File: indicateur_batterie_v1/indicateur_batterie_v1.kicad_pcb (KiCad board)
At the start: 2 copper layers, 28.5 x 16.5 mm, 13 parts, among them J1 Conn_01x02_Pin, Q1 Q_PMOS_GSD, U1 ATtiny412-SS, U3 MCP1802x-xx02xOT

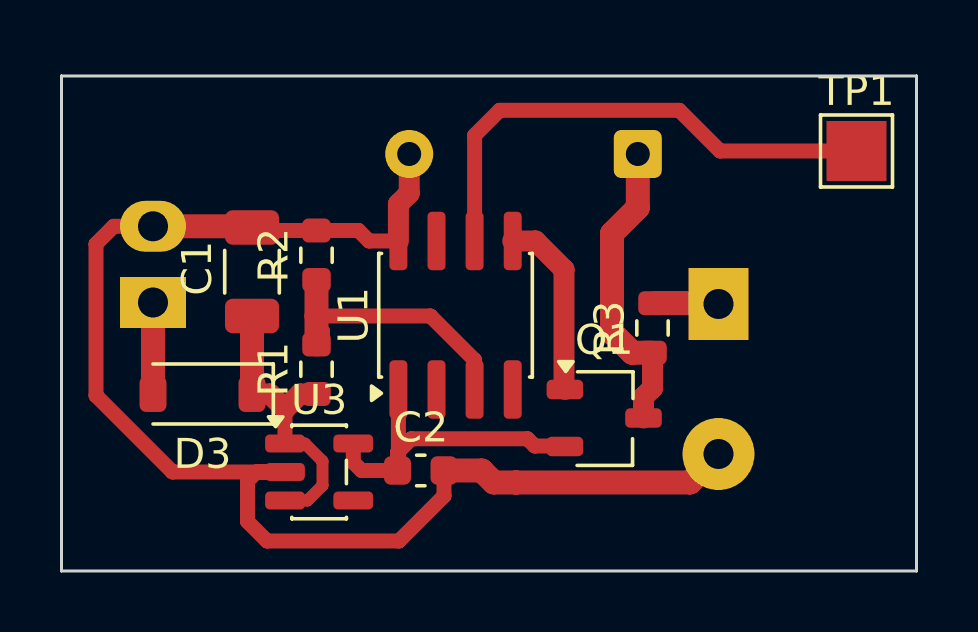
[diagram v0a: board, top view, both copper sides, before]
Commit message: changement déclanchement télécomande
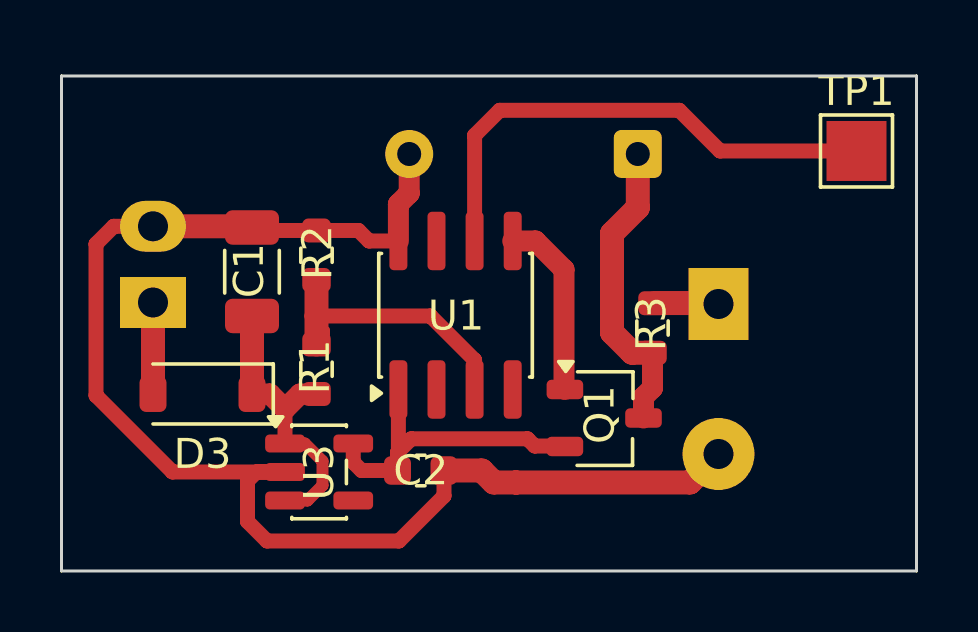
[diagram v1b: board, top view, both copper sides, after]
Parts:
- D3: value D_Schottky -> BAT54W D_Schottky
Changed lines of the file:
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@@
 		(tenting front back)
 		(pcbplotparams
-			(layerselection 0x00000000_00000000_55555555_55555551)
-			(plot_on_all_layers_selection 0x00000000_00000000_00000000_02000000)
+			(layerselection 0x00000000_00000000_55555555_57555550)
+			(plot_on_all_layers_selection 0x00000000_00000000_00000008_00000202)
 			(disableapertmacros no)
 			(usegerberextensions no)
@@
 			(subtractmaskfromsilk no)
 			(outputformat 4)
-			(mirror yes)
+			(mirror no)
 			(drillshape 1)
 			(scaleselection 1)
@@
 			)
 		)
-		(property "Value" "D_Schottky"
-			(at 0 2.1 0)
+		(property "Value" "BAT54W D_Schottky"
+			(at 9.2 0.1 0)
 			(layer "F.Fab")
 			(effects
@@
 		(tags "SOIC SO")
 		(property "Reference" "U1"
-			(at 0 -3.4 90)
+			(at -0.015 0.015 180)
 			(layer "F.SilkS")
 			(effects
@@
 		)
 		(property "Value" "ATtiny412-SS"
-			(at 0 3.4 90)
+			(at -9.265 1.705 90)
 			(layer "F.Fab")
 			(effects
@@
 		(tags "resistor")
 		(property "Reference" "R3"
-			(at 0 -1.43 90)
+			(at 0.14 -0.04 90)
 			(layer "F.SilkS")
 			(effects
@@
 		)
 		(property "Value" "0"
-			(at 0 1.43 90)
+			(at 2.13 0.04 90)
 			(layer "F.Fab")
 			(effects
@@
 		(tags "resistor")
 		(property "Reference" "R1"
-			(at 0 -1.43 90)
+			(at 0.075 -0.05 90)
 			(layer "F.SilkS")
 			(effects
@@
 		)
 		(property "Value" "10k"
-			(at 0 1.43 90)
+			(at 0.175 1.32 90)
 			(layer "F.Fab")
 			(effects
@@
 		(tags "capacitor")
 		(property "Reference" "C2"
-			(at 0 -1.43 0)
+			(at 0 0 0)
 			(layer "F.SilkS")
 			(effects
@@
 		(tags "SOT TO_SOT_SMD")
 		(property "Reference" "U3"
-			(at 0 -2.4 0)
+			(at 0 0.01 90)
 			(layer "F.SilkS")
 			(effects
@@
 		)
 		(property "Value" "MCP1802x-xx02xOT"
-			(at 0 2.4 0)
+			(at -0.0875 9.3 90)
 			(layer "F.Fab")
 			(effects
@@
 		(tags "capacitor")
 		(property "Reference" "C1"
-			(at 0.115 -1.83 90)
+			(at 0.035 -0.1 90)
 			(layer "F.SilkS")
 			(effects
@@
 		)
 		(property "Value" "10uF"
-			(at 0 1.85 90)
+			(at 4.205 0.04 90)
 			(layer "F.Fab")
 			(effects
@@
 		(tags "TSOT-23")
 		(property "Reference" "Q1"
-			(at 0 -2.6 0)
+			(at -0.15 -0.11 90)
 			(layer "F.SilkS")
 			(effects
@@
 		)
 		(property "Value" "Q_PMOS_GSD"
-			(at 0 2.5 0)
+			(at 0 7.1 90)
 			(layer "F.Fab")
 			(effects
@@
 		(tags "resistor")
 		(property "Reference" "R2"
-			(at 0 -1.43 90)
+			(at 0.085 0.03 90)
 			(layer "F.SilkS")
 			(effects
@@
 		)
 		(property "Value" "10k"
-			(at 0 1.43 90)
+			(at 2.855 -0.01 90)
 			(layer "F.Fab")
 			(effects
@@
 		(tags "buzzer")
 		(property "Reference" "BZ1"
-			(at 2.5 7.17 90)
+			(at 2.62 -2.82 180)
 			(layer "B.SilkS")
 			(effects
@@
 		(tags "Diode DO-35_SOD27 series Axial Horizontal pin pitch 7.62mm  length 4mm diameter 2mm")
 		(property "Reference" "D1"
-			(at 3.81 2.12 0)
+			(at 4.15 -0.04 0)
 			(layer "B.SilkS")
 			(effects
@@
 		)
 		(property "Value" "1N4148"
-			(at 3.86 -2.12 0)
+			(at 4.96 2.6 0)
 			(layer "B.Fab")
 			(effects
@@
 		)
 		(property "Value" "Conn_01x02_Pin"
-			(at 0 -5.31 0)
+			(at 0.16 -10.32 90)
 			(layer "B.Fab")
-			(effects
-				(font
+			(hide yes)
+			(effects
+				(font
